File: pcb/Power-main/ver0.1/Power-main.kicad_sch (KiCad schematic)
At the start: 8 parts, among them U1 LM5143QRHARQ1

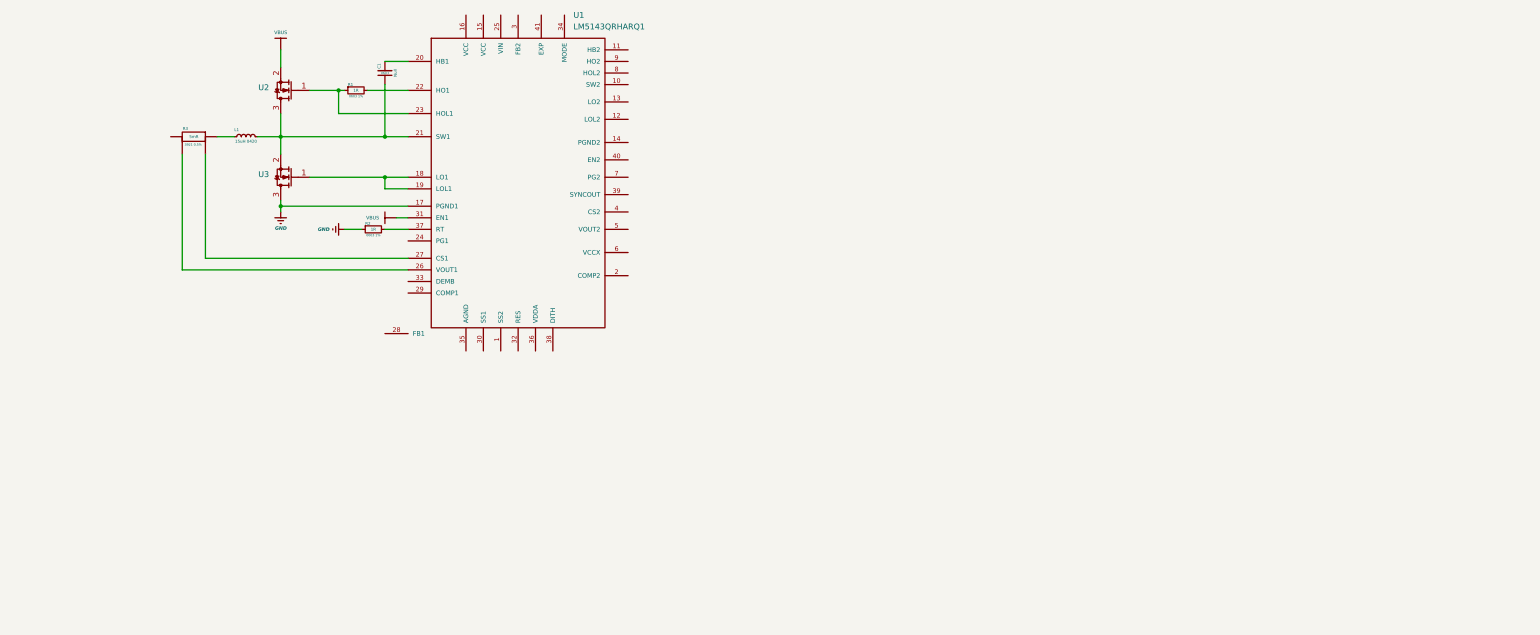
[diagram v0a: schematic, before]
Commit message: 主电源原理图
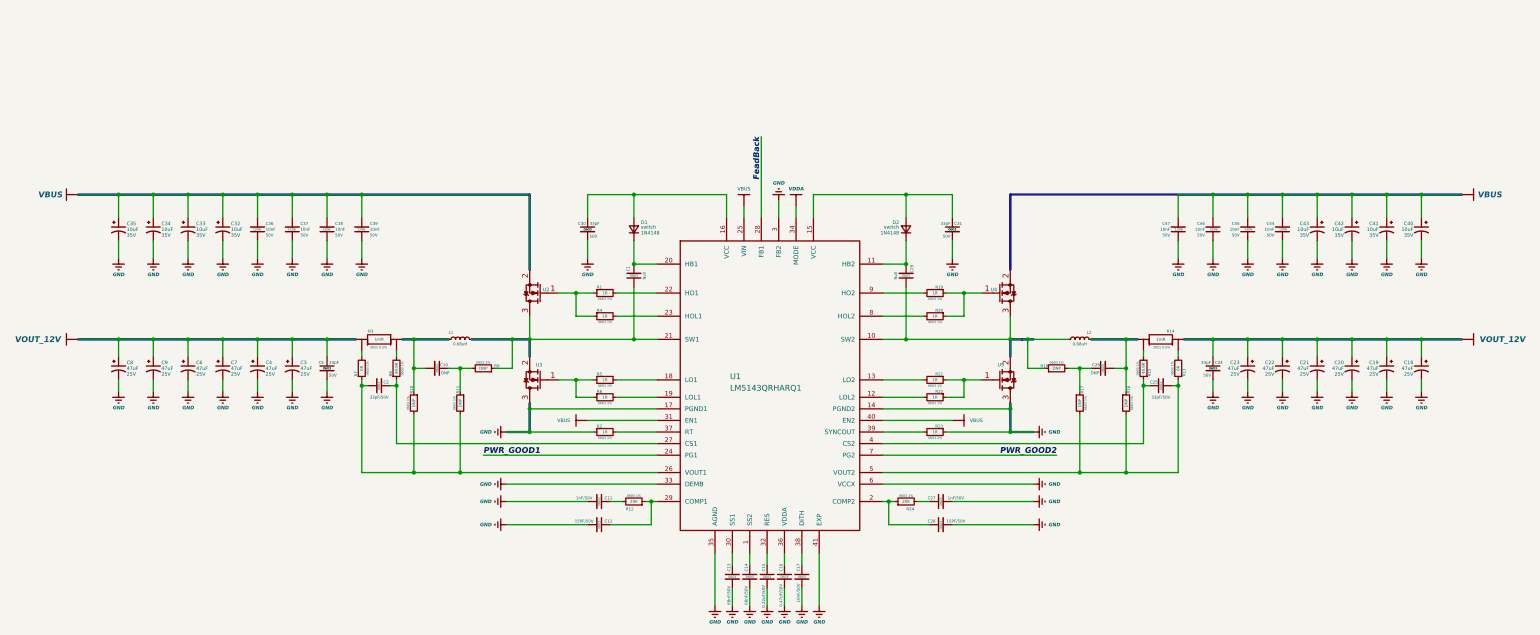
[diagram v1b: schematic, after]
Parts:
- added C10, C11, C12, C13, C14, C15, C16, C17, C2, C24, C25, C26, C27, C28, C29, C30, C31, C5: ~, Capacitor_SMD:C_0603_1608Metric, symbol Capacitor:C0603
- added C18, C19, C20, C21, C22, C23, C3, C32, C33, C34, C35, C4, C40, C41, C42, C43, C6, C7, C8, C9: 47uF 25V, symbol Capacitor:Cap
- added C36, C37, C38, C39, C44, C45, C46, C47: ~, 1206, symbol Capacitor:C1206
- added D1, D2: D_switch, symbol Diode_Symbol:D_switch
- added L2: 15uH, symbol Inductor:L_Small
- added R10, R11, R12, R13, R15, R16, R17, R18, R19, R20, R21, R22, R23, R24, R4, R5, R6, R7, R8, R9: ~, Resistor_SMD:R_0603_1608Metric, symbol Resistor:R0603
- added R14: 5mR 0.5%, symbol Resistor:R_Shunt_3920
- added U4, U5: ~, symbol MOSFET_Channel-N:Symbol-NMOS
- L1: Numeric&Footprint 15uH 0420 -> 0.68uH
- R3: Numeric 5mR -> 1mR
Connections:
- net GND: now also U1.14 (PGND2), U1.3 (FB2), U1.33 (DEMB), U1.35 (AGND), U1.41 (EXP), U1.6 (VCCX), C11.2, C12.2, C13.2, C14.2, C15.2, C16.2, C17.2, C18.2, C19.2, C20.2, C21.2, C22.2, C23.2, C24.2, C27.2, C28.2, C3.2, C30.2, C31.2, C32.2, C33.2, C34.2, C35.2, C36.1, C37.1, C38.1, C39.1, C4.2, C40.2, C41.2, C42.2, C43.2, C44.1, C45.1, C46.1, C47.1, C5.2, C6.2, C7.2, C8.2, C9.2, R23.1, U5.3
- net VBUS: now also U1.25 (VIN), U1.40 (EN2), C32.1, C33.1, C34.1, C35.1, C36.2, C37.2, C38.2, C39.2, C40.1, C41.1, C42.1, C43.1, C44.2, C45.2, C46.2, C47.2
- net at L1.1, R3.1: now also C10.2, R10.1
- net at U1.27 (CS1): now also C2.1, R8.1; no longer R3.2 (1)
- net at U1.26 (VOUT1): now also C2.2, R10.2, R11.2, R7.1; no longer R3.3 (2)
- net VOUT_12V: now reaches R3.4 (2)
- net VOUT_12V: now also C18.1, C19.1, C20.1, C21.1, C22.1, C23.1, C24.1, C3.1, C4.1, C5.1, C6.1, C7.1, C8.1, C9.1, R14.4 (2)
- net at C1.1, L1.2, U1.21 (SW1)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: now also R9.1
- net at C1.2, U1.20 (HB1): now also D1.1 (K)
- net at R1.1, U2.1: now also R4.1; no longer U1.23 (HOL1)
- net at U1.1 (SS2): now also C14.1
- net at U1.10 (SW2): now also C29.1, L2.2, R18.1, U4.3, U5.2
- net at U1.11 (HB2): now also C29.2, D2.1 (K)
- net at U1.12 (LOL2): now also R22.2
- net at U1.13 (LO2): now also R21.2
- net at U1.15 (VCC): now also C31.1, D2.2 (A)
- net at U1.16 (VCC): now also C30.1, D1.2 (A)
- net at U1.2 (COMP2): now also C28.1, R24.1
- net PWR_GOOD1: now reaches U1.24 (PG1)
- net FeadBack: now reaches U1.28 (FB1)
- net at U1.29 (COMP1): now also C12.1, R12.1
- net at U1.30 (SS1): now also C13.1
- net at U1.32 (RES): now also C15.1
- net VDDA: now reaches U1.34 (MODE)
- net at U1.36 (VDDA): now also C16.1
- net at U1.38 (DITH): now also C17.1
- net at U1.39 (SYNCOUT): now also R23.2
- net at U1.4 (CS2): now also C25.1, R15.1
- net at U1.5 (VOUT2): now also C25.2, R13.1, R16.2, R17.2
- net PWR_GOOD2: now reaches U1.7 (PG2)
- net at U1.8 (HOL2): now also R20.2
- net at U1.9 (HO2): now also R19.2
- new net: C27.1, R24.2
- new net: R14.2 (1), R15.2
- new net: C11.1, R12.2
- new net: C10.1, R11.1, R9.2
- new net: R5.1, R6.1, U3.1
- new net: R5.2, U1.18 (LO1)
- new net: R3.2 (1), R8.2
- new net: R3.3 (2), R7.2
- new net: R6.2, U1.19 (LOL1)
- new net: R4.2, U1.23 (HOL1)
- new net: R21.1, R22.1, U5.1
- new net: R19.1, R20.1, U4.1
- new net: C26.1, R17.1, R18.2
- new net: C26.2, L2.1, R14.1, R16.1
- new net: R13.2, R14.3 (2)
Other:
- company: (none) -> Item
- title: (none) -> LM5143测试板
- moved on the sheet: C1, L1, R1, R2, R3, U1, U3
